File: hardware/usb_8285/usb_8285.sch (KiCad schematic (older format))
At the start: 24 parts, among them P1 UTX, P10 ADC, P2 URX, P3 D+, P4 +5V, P5 +5V, P6 GND, P7 GND, P8 D-, P9 G0, U1 ESP8285, U2 1824, X1 26MHz

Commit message: update hardware - yes, it works!
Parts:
- A1, R1, R2, R5: symbol R -> R-RESCUE-usb_8285
- C1, C2, C3, C4, C5, C6: symbol C -> C-RESCUE-usb_8285
- R4: value 1.5k -> NOPOP; symbol R -> R-RESCUE-usb_8285
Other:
- note added: "TESTED WORKING 2016-08-26 C.L."
- note removed: "UNTESTED DO NOT USE"
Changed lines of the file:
@@
 LIBS:memory
 LIBS:xilinx
-LIBS:special
 LIBS:microcontrollers
 LIBS:dsp
@@
 LIBS:lsm303d
 LIBS:lsm303c
+LIBS:lsm9ds1
 LIBS:lsm9ds0
 LIBS:lm386
@@
 LIBS:2.4GHZ_2450FB15L0001
 LIBS:usb_8285-cache
-EELAYER 27 0
+EELAYER 25 0
 EELAYER END
 $Descr USLetter 11000 8500
@@
 $EndComp
 $Comp
-L GND #PWR01
+L GND-RESCUE-usb_8285 #PWR01
 U 1 1 57A25A3B
 P 4100 1600
@@
 	4300 1600 4300 1400
 $Comp
-L R R1
+L R-RESCUE-usb_8285 R1
 U 1 1 57A25A68
 P 4050 1400
@@
 $EndComp
 $Comp
-L C C3
+L C-RESCUE-usb_8285 C3
 U 1 1 57A25A83
 P 3050 2150
@@
 	3250 2150 3400 2150
 $Comp
-L +3.3V #PWR02
+L +3.3V-RESCUE-usb_8285 #PWR02
 U 1 1 57A25AA5
 P 4500 1450
@@
 Connection ~ 4500 1500
 $Comp
-L +3.3V #PWR03
+L +3.3V-RESCUE-usb_8285 #PWR03
 U 1 1 57A25ABA
 P 3400 2050
@@
 $EndComp
 $Comp
-L GND #PWR04
+L GND-RESCUE-usb_8285 #PWR04
 U 1 1 57A25AC0
 P 3800 1400
@@
 $EndComp
 $Comp
-L GND #PWR05
+L GND-RESCUE-usb_8285 #PWR05
 U 1 1 57A25AD5
 P 4750 1100
@@
 	4450 1050 4450 750
 $Comp
-L C C1
+L C-RESCUE-usb_8285 C1
 U 1 1 57A25B1A
 P 4150 900
@@
 $EndComp
 $Comp
-L C C2
+L C-RESCUE-usb_8285 C2
 U 1 1 57A25B20
 P 5400 1000
@@
 $EndComp
 $Comp
-L GND #PWR06
+L GND-RESCUE-usb_8285 #PWR06
 U 1 1 57A25B26
 P 3950 900
@@
 Connection ~ 4450 900
 $Comp
-L GND #PWR07
+L GND-RESCUE-usb_8285 #PWR07
 U 1 1 57A25B3F
 P 5600 1000
@@
 Connection ~ 5150 1000
 $Comp
-L +3.3V #PWR08
+L +3.3V-RESCUE-usb_8285 #PWR08
 U 1 1 57A25B5A
 P 3400 2650
@@
 $EndComp
 $Comp
-L +3.3V #PWR09
+L +3.3V-RESCUE-usb_8285 #PWR09
 U 1 1 57A25B60
 P 5550 2750
@@
 $EndComp
 $Comp
-L +3.3V #PWR010
+L +3.3V-RESCUE-usb_8285 #PWR010
 U 1 1 57A25B66
 P 3400 2350
@@
 $EndComp
 $Comp
-L +3.3V #PWR011
+L +3.3V-RESCUE-usb_8285 #PWR011
 U 1 1 57A25B76
 P 3400 2250
@@
 	3400 2550 3000 2550
 $Comp
-L +3.3V #PWR012
+L +3.3V-RESCUE-usb_8285 #PWR012
 U 1 1 57A25D5E
 P 4400 3200
@@
 $EndComp
 $Comp
-L GND #PWR013
+L GND-RESCUE-usb_8285 #PWR013
 U 1 1 57A25D64
 P 4600 3200
@@
 $EndComp
 $Comp
-L C C4
+L C-RESCUE-usb_8285 C4
 U 1 1 57A25EB1
 P 2350 2550
@@
 $EndComp
 $Comp
-L C C5
+L C-RESCUE-usb_8285 C5
 U 1 1 57A25EB7
 P 2600 2550
@@
 $EndComp
 $Comp
-L GND #PWR014
+L GND-RESCUE-usb_8285 #PWR014
 U 1 1 57A26375
 P 6500 3300
@@
 	4800 3500 4800 3200
 $Comp
-L +3.3V #PWR015
+L +3.3V-RESCUE-usb_8285 #PWR015
 U 1 1 57A26412
 P 4250 3400
@@
 $EndComp
 $Comp
-L R R2
+L R-RESCUE-usb_8285 R2
 U 1 1 57A26418
 P 4500 3400
@@
 $EndComp
 $Comp
-L GND #PWR017
+L GND-RESCUE-usb_8285 #PWR017
 U 1 1 57A26482
 P 6850 2800
@@
 $EndComp
 $Comp
-L +3.3V #PWR019
+L +3.3V-RESCUE-usb_8285 #PWR019
 U 1 1 57A2648E
 P 2350 2350
@@
 $EndComp
 $Comp
-L +3.3V #PWR020
+L +3.3V-RESCUE-usb_8285 #PWR020
 U 1 1 57A26494
 P 2600 2350
@@
 $EndComp
 $Comp
-L GND #PWR021
+L GND-RESCUE-usb_8285 #PWR021
 U 1 1 57A2649A
 P 2450 2850
@@
 $EndComp
 $Comp
-L GND #PWR023
+L GND-RESCUE-usb_8285 #PWR023
 U 1 1 57A264F8
 P 1750 3850
@@
 $EndComp
 $Comp
-L +3.3V #PWR025
+L +3.3V-RESCUE-usb_8285 #PWR025
 U 1 1 57A26504
 P 2950 3750
@@
 $EndComp
 $Comp
-L C C6
+L C-RESCUE-usb_8285 C6
 U 1 1 57A26510
 P 1400 3950
@@
 $EndComp
 $Comp
-L GND #PWR027
+L GND-RESCUE-usb_8285 #PWR027
 U 1 1 57A26516
 P 1400 4150
@@
 	1    0    0    -1
 $EndComp
-Text Notes 2100 5650 0    394  ~ 0
-UNTESTED DO NOT USE
-$Comp
-L R A1
+Text Notes 3800 4450 0    236  ~ 0
+TESTED WORKING 2016-08-26 C.L.
+$Comp
+L R-RESCUE-usb_8285 A1
 U 1 1 57A8E837
 P 2850 1900
@@
 $EndComp
 $Comp
-L GND #PWR028
+L GND-RESCUE-usb_8285 #PWR028
 U 1 1 57A8F089
 P 4200 3200
@@
 $EndComp
 $Comp
-L GND #PWR029
+L GND-RESCUE-usb_8285 #PWR029
 U 1 1 57A8F08F
 P 4300 3200
@@
 $EndComp
 $Comp
-L R R4
+L R-RESCUE-usb_8285 R4
 U 1 1 57A8F4F8
 P 6500 2200
 F 0 "R4" V 6580 2200 40  0000 C CNN
-F 1 "1.5k" V 6507 2201 40  0000 C CNN
+F 1 "NOPOP" V 6507 2201 40  0000 C CNN
 F 2 "SM0603" V 6430 2200 30  0000 C CNN
 F 3 "~" H 6500 2200 30  0000 C CNN
@@
 D+
 $Comp
-L R R5
+L R-RESCUE-usb_8285 R5
 U 1 1 57A8F67C
 P 5300 3700
@@
 $EndComp
 $Comp
-L +3.3V #PWR030
+L +3.3V-RESCUE-usb_8285 #PWR030
 U 1 1 57A8F682
 P 5550 3700
@@
 $EndComp
 $Comp
-L +3.3V #PWR031
+L +3.3V-RESCUE-usb_8285 #PWR031
 U 1 1 57B211DF
 P 6750 2200

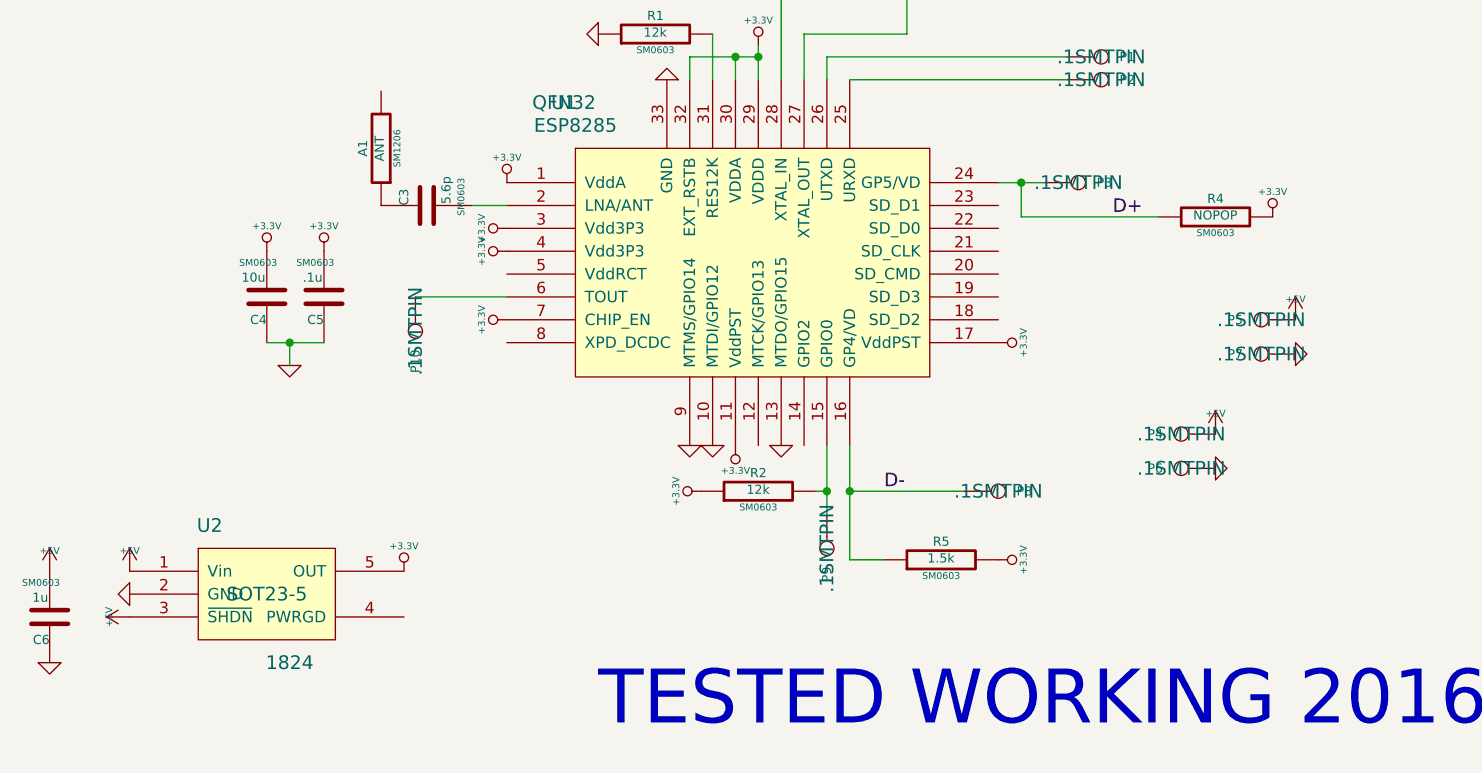
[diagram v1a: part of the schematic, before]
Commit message: fix layout
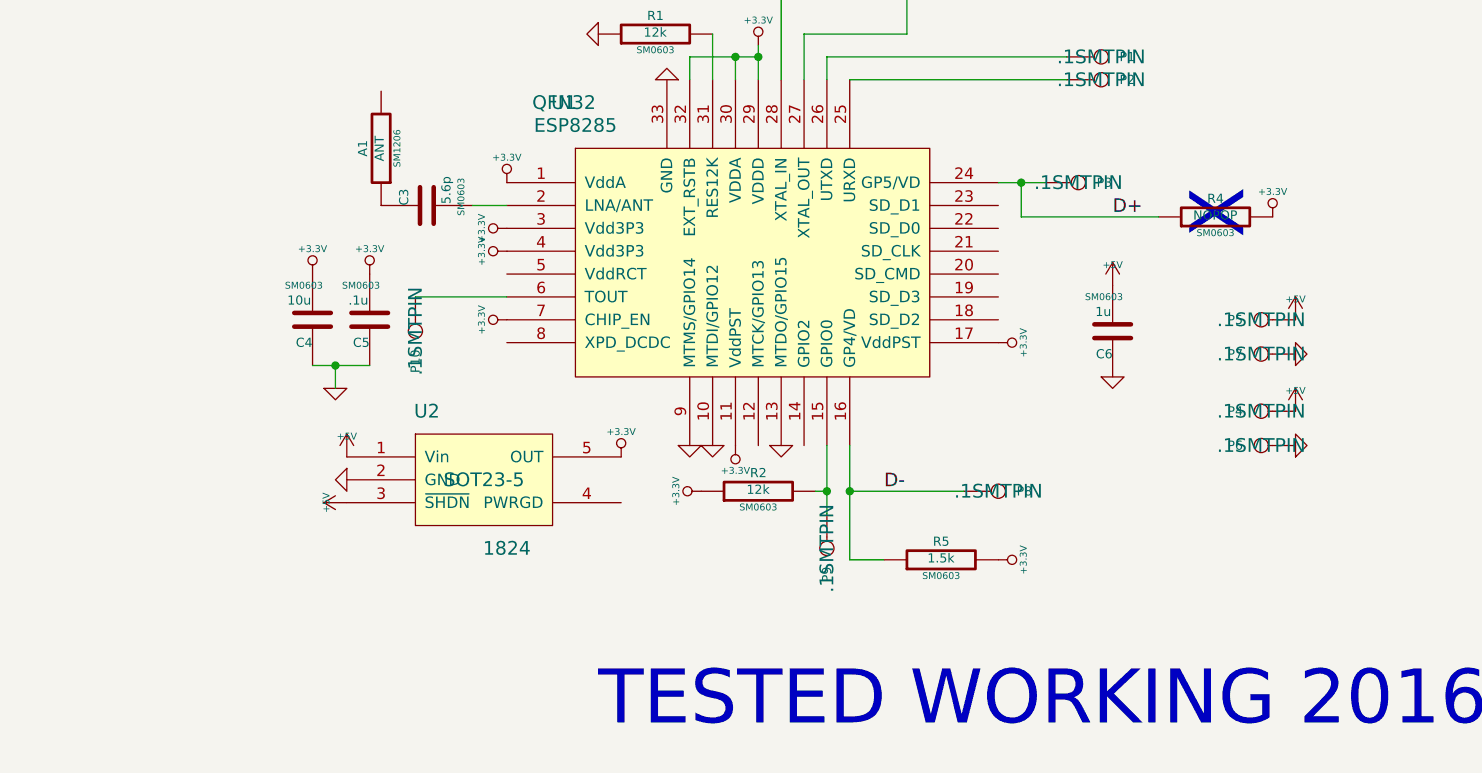
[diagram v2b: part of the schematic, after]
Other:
- note added: "X"
- moved on the sheet: C4, C5, C6, P4, P6, U2
